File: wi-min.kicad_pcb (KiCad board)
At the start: 2 copper layers, 44.4 x 29.2 mm, 6 parts, among them CON1 AVR-ISP-6, IC1 ATMEGA8A-P, P1 BAT_3V, P2 NRF24_CONN_5X2, P3 CONN_4

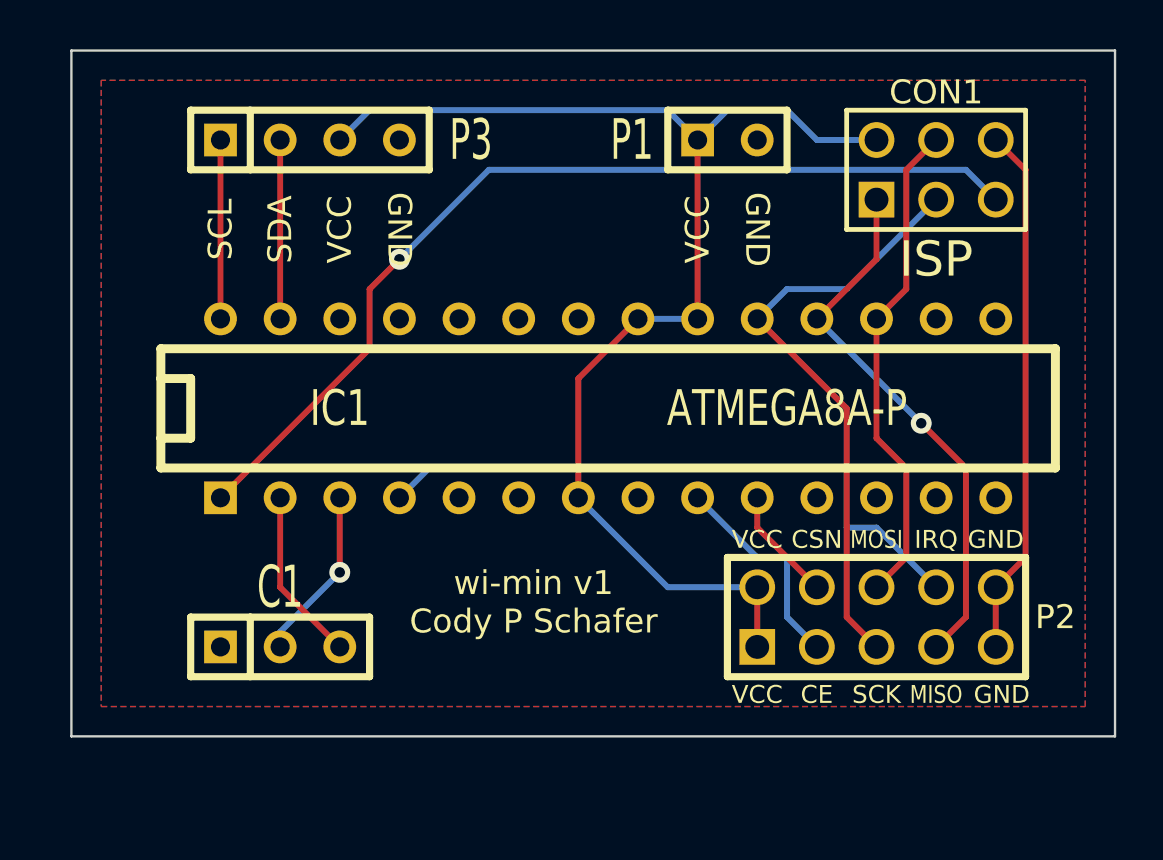
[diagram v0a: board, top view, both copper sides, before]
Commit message: post v2
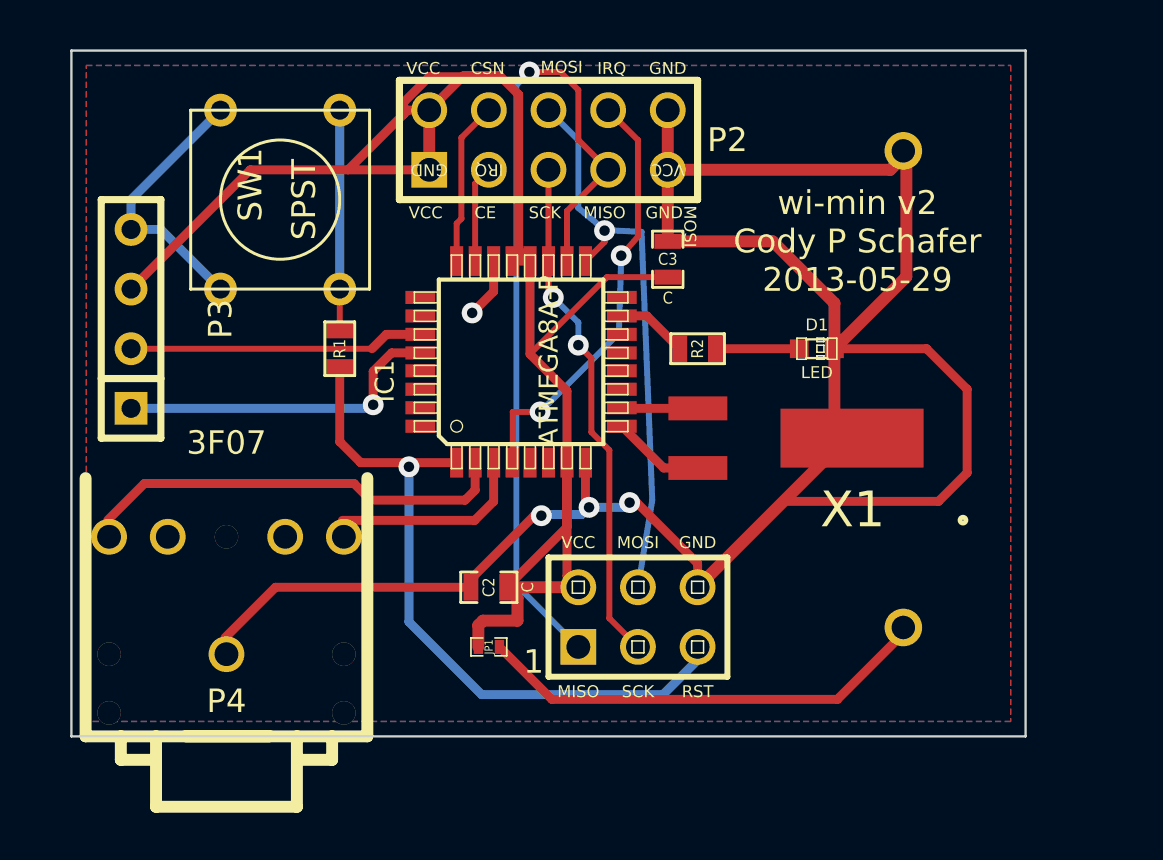
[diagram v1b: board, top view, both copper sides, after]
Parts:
- removed C1: SERIAL_TTL_3.5MM, SIL-3
- added C2: C, SM0603_Capa, F.Cu at (198.1, 119.4)
- added C3: C, SM0603_Capa, F.Cu at (205.7, 105.4)
- added D1: LED, LED-0603, F.Cu at (212.1, 109.2)
- added JP1: JUMPER, SM0402, F.Cu at (198.1, 121.9)
- added P4: 3F07, 3F07, F.Cu at (186.9, 125.7)
- added R1: R, SM0603, F.Cu at (191.8, 109.2)
- added R2: R, SM0603, F.Cu at (207.0, 109.2)
- added SW1: SPST, SW_PUSH_SMALL, F.Cu at (189.2, 102.9)
- added X1: CRYSTAL_W_GND, AB26TRB, F.Cu at (208.3, 113.0)
- CON1: footprint pin_array_3x2 -> atmel-2-AVR-ISP-6
- IC1: footprint DIP-28__300 -> atmel-TQFP32
- P1: value BAT_3V -> BATTERY; footprint SIL-2 -> CR2032_HOLDER_TH; moved to B.Cu
- moved P2 24.7 mm to (200.7, 100.3)
- moved CON1 22.9 mm to (204.5, 120.7)
- moved P1 11.5 mm to (215.8, 109.1)
- moved P3 10.8 mm to (182.9, 108.0), turned to 90 degrees
- moved IC1 4.20 mm to (199.5, 109.8), turned to 90 degrees
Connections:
- net /INT0 renamed /IRQ
- IC1 pad 10: N-000005 -> /TOSC2
- IC1 pad 15: (no net) -> /DBG_LED
- IC1 pad 2: /Rx -> /Tx
- IC1 pad 23: (no net) -> /CE
- IC1 pad 24: (no net) -> /CSN
- IC1 pad 3: /Tx -> /Rx
- IC1 pad 9: N-000009 -> /TOSC1
- P1 pad 1: VCC -> N-0000012
- P2 pad 3: N-000009 -> /CE
- P2 pad 4: N-000005 -> /CSN
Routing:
- net GND: track 22.6 -> 113.5 mm, vias 0 -> 4
- net N-0000012: track 0.00 -> 19.5 mm
- net VCC: track 55.5 -> 74.1 mm
- net /MISO: track 23.3 -> 36.8 mm
- net /RST: track 40.8 -> 30.1 mm
- net /Tx: track 7.40 -> 17.9 mm, vias 1 -> 0
- net N-000001: track 0.00 -> 9.40 mm
- net N-000009: track 9.20 -> 0.00 mm
- net /IRQ: track 27.0 -> 18.4 mm, vias 0 -> 2
- net /CSN: track 0.00 -> 6.99 mm
- net /SCL: track 7.62 -> 14.1 mm, vias 0 -> 1
- net /SDA: track 7.62 -> 12.6 mm
- net N-000005: track 4.86 -> 0.00 mm
- net /CE: track 0.00 -> 4.13 mm
- net /TOSC1: track 0.00 -> 3.97 mm
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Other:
- board size 44.4 x 29.2 mm -> 40.6 x 29.2 mm
- net class Minimal added: clearance 0.1524, trace_width 0.1524, via_dia 0.508, via_drill 0.3302
- rule trace_min: 0.254 -> 0.1524
- rule via_min_drill: 0.508 -> 0.3302
- rule via_min_size: 0.889 -> 0.508
- board text added: "wi-min v2 Cody P Schafer 2013-05-29"
- board text removed: "ISP"
- board text removed: "SCL"
- board text removed: "SDA"
- board text removed: "wi-min v1 Cody P Schafer"

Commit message: v3 sent for fabrication
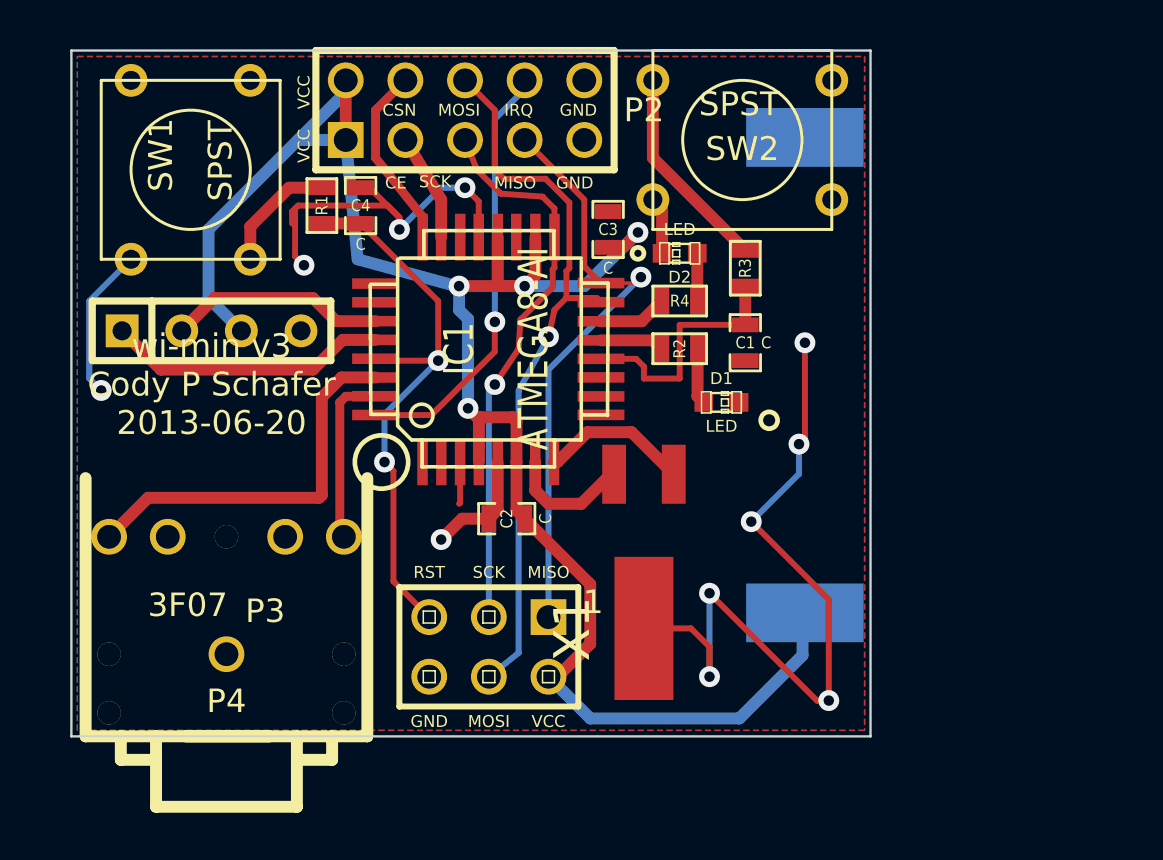
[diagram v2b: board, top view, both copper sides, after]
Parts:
- removed JP1: JUMPER, SM0402
- added C1: C, SM0603_Capa, F.Cu at (209.0, 109.0)
- added C4: C, SM0603_Capa, F.Cu at (192.7, 103.1)
- added D2: LED, LED-0603, F.Cu at (206.2, 105.2)
- added R3: R, SM0603, F.Cu at (209.0, 105.8)
- added R4: 150R, SM0603, F.Cu at (206.2, 107.2)
- added SW2: SPST, SW_PUSH_SMALL, F.Cu at (208.9, 100.3)
- IC1: value ATMEGA8A-P -> ATMEGA8-AI; footprint atmel-TQFP32 -> TQFP32
- P1: footprint CR2032_HOLDER_TH -> CR2032_HOLDER_TH_ON_SIDE
- R2: value R -> 150R
- moved CON1 6.48 mm to (198.1, 121.9), turned to 180 degrees
- moved R1 6.14 mm to (191.0, 103.1)
- moved D1 4.66 mm to (208.0, 111.5)
- moved X1 4.52 mm to (204.7, 115.8), turned to 90 degrees
- moved P1 4.19 mm to (211.6, 109.2)
- moved SW1 4.02 mm to (185.4, 101.6)
- moved P2 3.78 mm to (197.1, 99.1)
- moved P3 3.47 mm to (186.3, 108.5), turned to 0 degrees
- moved C2 3.02 mm to (198.9, 116.5)
- moved C3 2.84 mm to (203.2, 104.1)
- moved IC1 1.48 mm to (198.1, 109.2)
- moved R2 0.76 mm to (206.2, 109.2)
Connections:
- IC1 pad 1: /RST -> (no net)
- IC1 pad 10: /TOSC2 -> (no net)
- IC1 pad 12: (no net) -> /USR_BUTTON
- IC1 pad 13: (no net) -> /LED0
- IC1 pad 14: (no net) -> /LED1
- IC1 pad 15: /DBG_LED -> /MOSI
- IC1 pad 16: (no net) -> /MISO
- IC1 pad 17: /MOSI -> /SCK
- IC1 pad 18: /MISO -> VCC
- IC1 pad 19: /SCK -> (no net)
- IC1 pad 2: /Tx -> (no net)
- IC1 pad 21: VCC -> GND
- IC1 pad 22: GND -> (no net)
- IC1 pad 29: (no net) -> /RST
- IC1 pad 3: /Rx -> GND
- IC1 pad 30: (no net) -> /Tx
- IC1 pad 31: (no net) -> /Rx
- IC1 pad 32: (no net) -> /IRQ
- IC1 pad 4: /IRQ -> VCC
- IC1 pad 5: (no net) -> GND
- IC1 pad 6: (no net) -> VCC
- IC1 pad 7: VCC -> /TOSC1
- IC1 pad 8: GND -> /TOSC2
- IC1 pad 9: /TOSC1 -> (no net)
- P1 pad 1: N-0000012 -> VCC
- R2 pad 1: /DBG_LED -> /LED0
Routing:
- net GND: track 113.5 -> 64.8 mm, vias 4 -> 11
- net /MISO: track 36.8 -> 25.4 mm
- net /USR_BUTTON: track 0.00 -> 10.7 mm
- net N-0000012: track 19.5 -> 8.87 mm
- net VCC: track 74.1 -> 80.7 mm, vias 0 -> 4
- net /MOSI: track 24.6 -> 31.1 mm
- net /RST: track 30.1 -> 24.2 mm, vias 1 -> 2
- net N-0000030: track 9.40 -> 5.13 mm
- net /SDA: track 12.6 -> 9.24 mm
- net /TOSC2: track 3.25 -> 6.36 mm
- net /DBG_LED: track 3.04 -> 0.00 mm
- net /LED1: track 0.00 -> 2.95 mm
- net /LED0: track 0.00 -> 2.74 mm
- net /SCL: track 14.1 -> 12.0 mm, vias 1 -> 0
- net N-0000014: track 0.00 -> 2.04 mm
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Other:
- board size 40.6 x 29.2 mm -> 34 x 29.2 mm
- board text added: "wi-min v3 Cody P Schafer 2013-06-20"
- board text removed: "wi-min v2 Cody P Schafer 2013-05-29"
